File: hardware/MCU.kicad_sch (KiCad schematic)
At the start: 13 parts, among them SW10 SW_Push, SW4 SW_Push, SW6 SW_Push, SW7 SW_Push, SW8 SW_Push, SW9 SW_Push

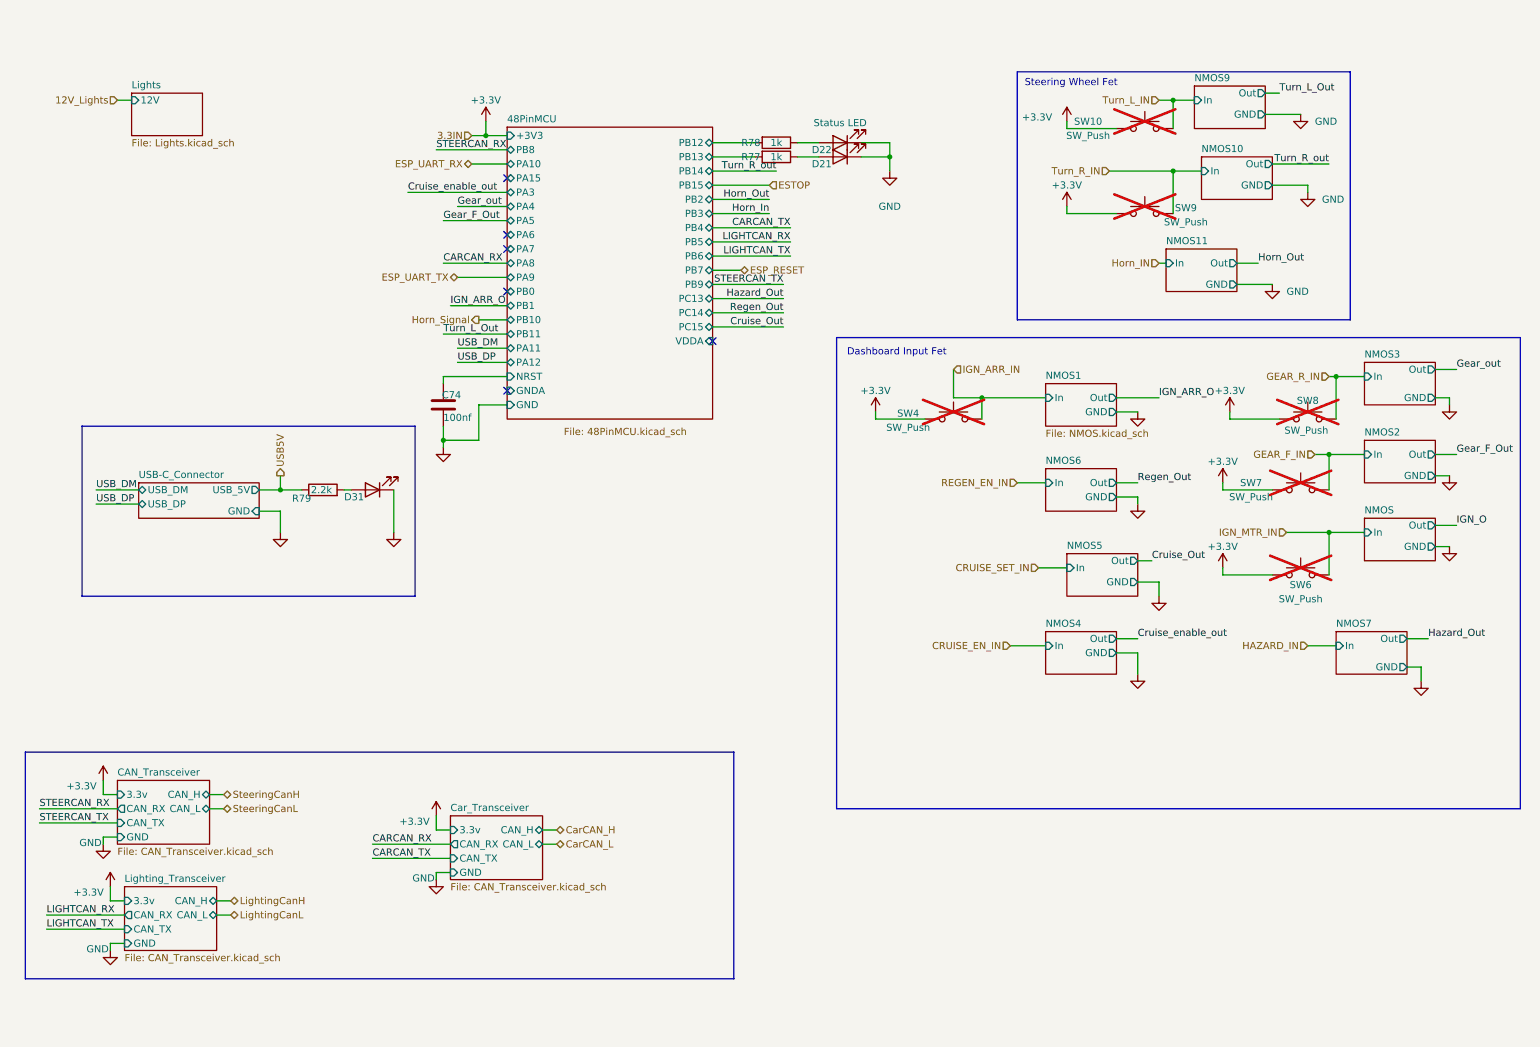
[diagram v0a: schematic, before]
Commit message: rawr
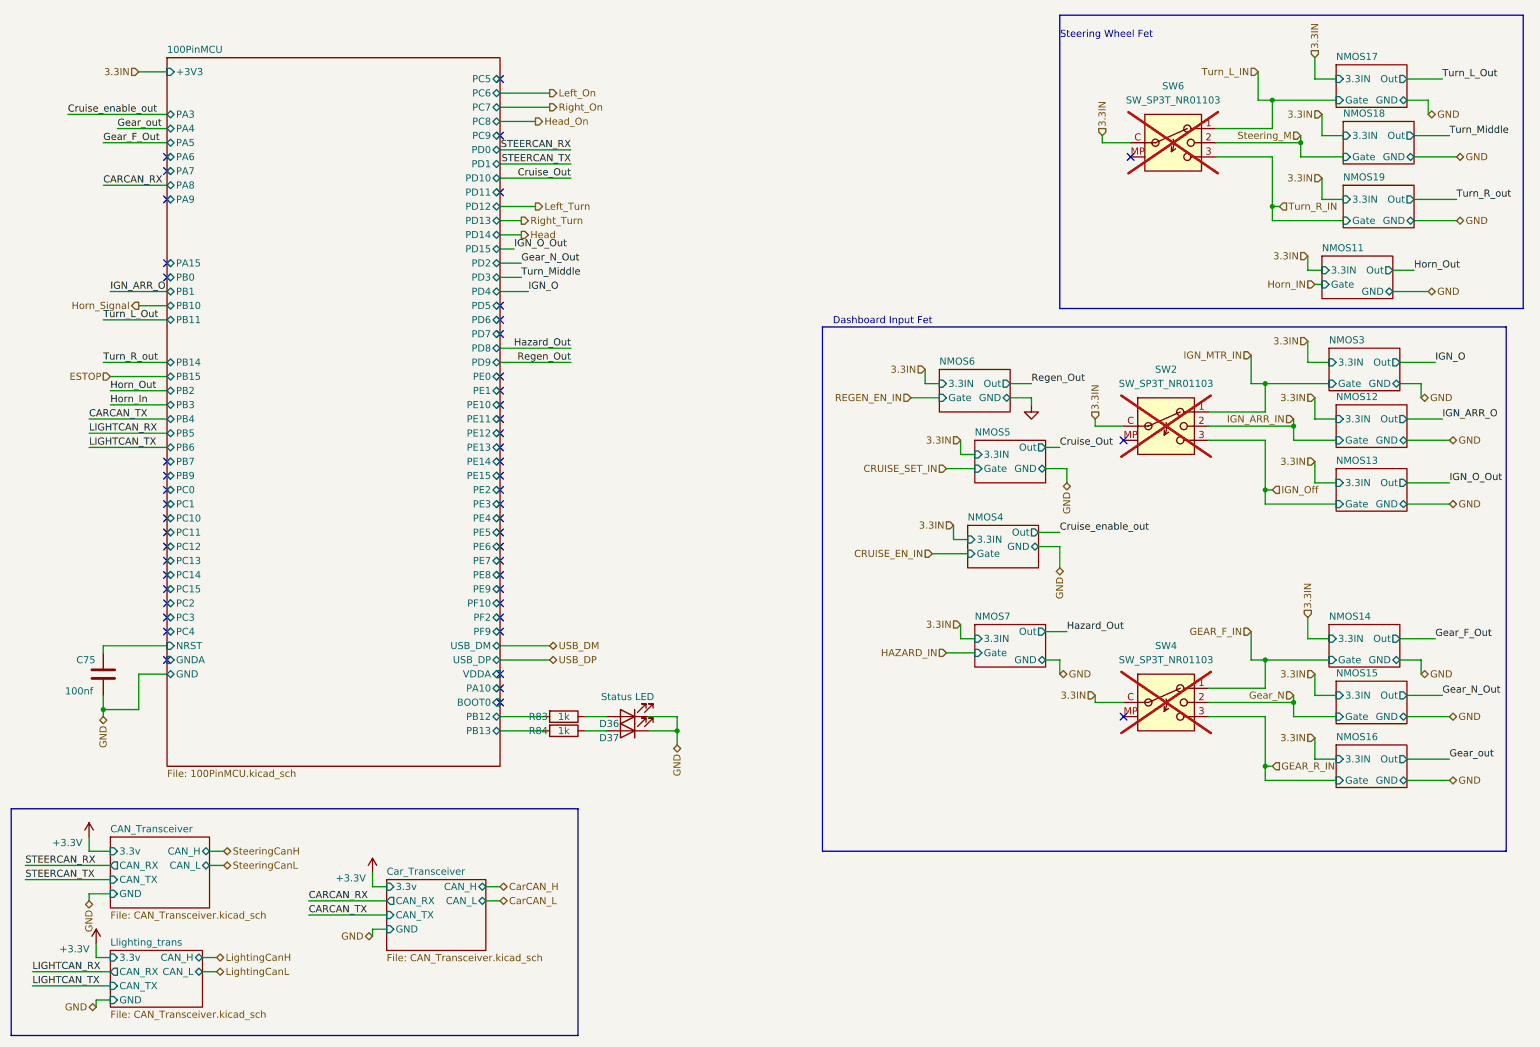
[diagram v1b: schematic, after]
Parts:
- removed C74: 100nf, symbol Device:C
- removed D21, D22, D31: Status LED, symbol Device:LED
- removed R77, R78: 1k, symbol Device:R
- removed R79: 2.2k, symbol Device:R
- removed SW10, SW4, SW6, SW7, SW8, SW9: SW_Push, symbol Switch:SW_Push
- added C75: 100nf, symbol Device:C
- added D36, D37: Status LED, symbol Device:LED
- added R83, R84: 1k, symbol Device:R
- added SW2, SW4, SW6: SW_SP3T_NR01103, Button_Switch_THT:SW_NKK_NR01, symbol Switch:SW_SP3T_NR01103
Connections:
- net GEAR_F_IN: now also SW4.1
- net GEAR_R_IN: now also SW4.3
- net GND: now also C75.2, D36.1 (K), D37.1 (K)
- net IGN_ARR_IN: now also SW2.2
- net IGN_MTR_IN: now also SW2.1
- net Turn_L_IN: now also SW6.1
- net Turn_R_IN: now also SW6.3
- new net: D36.2 (A), R83.1
- new net: D37.2 (A), R84.1
- new net 100PinMCU/NRST: C75.1
- new net 100PinMCU/PB12: R83.2
- new net 100PinMCU/PB13: R84.2
- new net 3.3IN: SW2.C (Common), SW4.C (Common), SW6.C (Common)
- new net Gear_N: SW4.2
- new net IGN_Off: SW2.3
- new net Steering_M: SW6.2
- no-connect marks 6 -> 50
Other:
- removed sheet 48PinMCU
- removed sheet Lighting_Transceiver
- removed sheet Lights
- removed sheet NMOS
- removed sheet NMOS1
- removed sheet NMOS10
- removed sheet NMOS2
- removed sheet NMOS9
- removed sheet USB-C_Connector
- added sheet 100PinMCU (100PinMCU.kicad_sch)
- added sheet Llighting_trans (CAN_Transceiver.kicad_sch)
- added sheet NMOS12 (NMOS.kicad_sch)
- added sheet NMOS13 (NMOS.kicad_sch)
- added sheet NMOS14 (NMOS.kicad_sch)
- added sheet NMOS15 (NMOS.kicad_sch)
- added sheet NMOS16 (NMOS.kicad_sch)
- added sheet NMOS17 (NMOS.kicad_sch)
- added sheet NMOS18 (NMOS.kicad_sch)
- added sheet NMOS19 (NMOS.kicad_sch)
- sheet NMOS11 ports: added 3.3IN, Gate; removed In
- sheet NMOS3 ports: added 3.3IN, Gate; removed In
- sheet NMOS4 ports: added 3.3IN, Gate; removed In
- sheet NMOS5 ports: added 3.3IN, Gate; removed In
- sheet NMOS6 ports: added 3.3IN, Gate; removed In
- sheet NMOS7 ports: added 3.3IN, Gate; removed In
